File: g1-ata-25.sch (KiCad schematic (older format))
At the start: 29 parts, among them P1 G1_DC_SOCKET, P2 G1_GD_PLUGNH, P3 IDE_40PIN, P4 IDE_44PIN, P5 CONN_01X02, P6 CONN_01X04, P7 BARREL_JACK, P8 CONN_01X05, U1 TCXO_DFAS11, U2 TS30011-M050

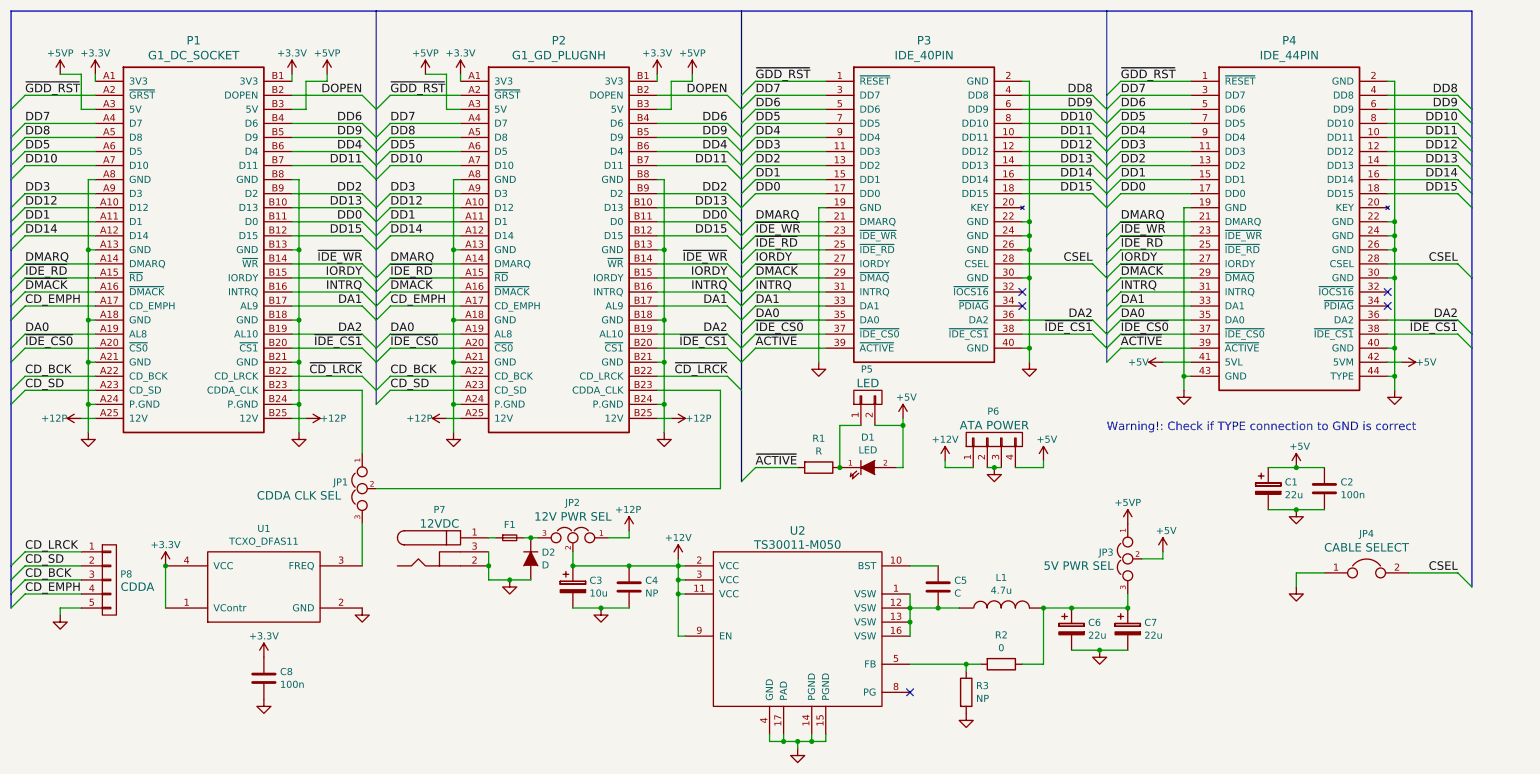
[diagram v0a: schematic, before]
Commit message: First test placing components.
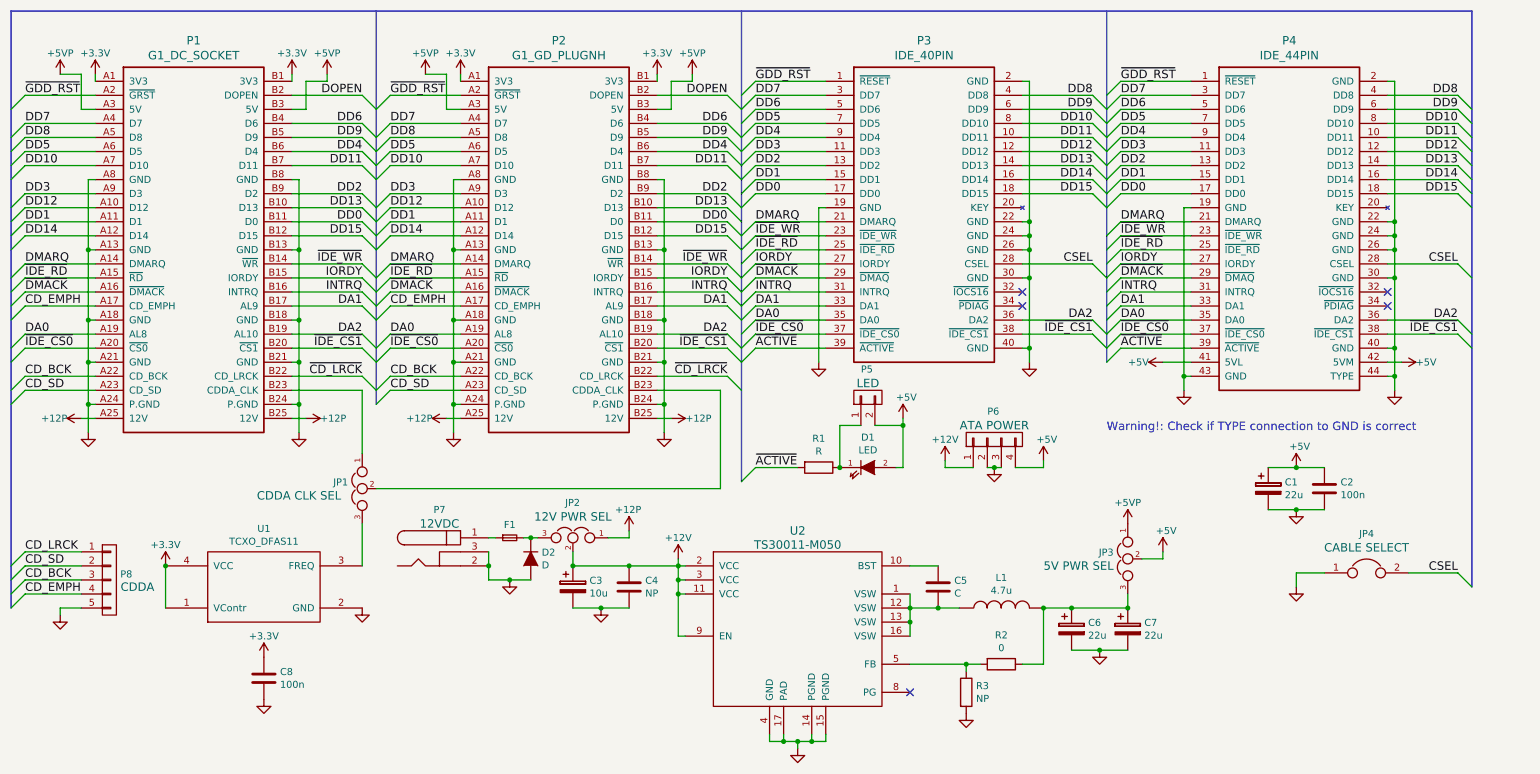
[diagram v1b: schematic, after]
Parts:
- C1, C6, C7, L1: footprint (none) -> Capacitors_SMD:C_1206
- C2, C3, C4, C5, C8, F1: footprint (none) -> Capacitors_SMD:C_0805
- D1: footprint (none) -> LEDs:LED_0603
- D2: footprint (none) -> Diodes_SMD:MiniMELF_Standard
- JP1, JP2, JP3: footprint (none) -> Pin_Headers:Pin_Header_Straight_1x03
- JP4: footprint (none) -> Pin_Headers:Pin_Header_Straight_1x02
- P1: footprint (none) -> doragasu:MOLEX_53408-0570
- P2: footprint (none) -> doragasu:MOLEX_52584-0508
- P3: footprint (none) -> Socket_Strips:Socket_Strip_Straight_2x20
- P4: footprint (none) -> doragasu:SOCKET_2X22_2MM_ANGLE
- P5: footprint (none) -> Socket_Strips:Socket_Strip_Straight_1x02
- P6: footprint (none) -> Socket_Strips:Socket_Strip_Straight_1x04
- P7: footprint (none) -> Connect:BARREL_JACK
- P8: footprint (none) -> Socket_Strips:Socket_Strip_Straight_1x05
- R1, R2, R3: footprint (none) -> Resistors_SMD:R_0805
- U1: footprint (none) -> doragasu:OSC_F530L
- U2: footprint (none) -> Housings_DFN_QFN:QFN-16-1EP_3x3mm_Pitch0.5mm
